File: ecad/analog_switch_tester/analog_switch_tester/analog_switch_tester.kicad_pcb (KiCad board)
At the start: 2 copper layers, 5 parts, among them J1 Conn_01x03_Pin, U1 DRV5056A1xQDBZxR

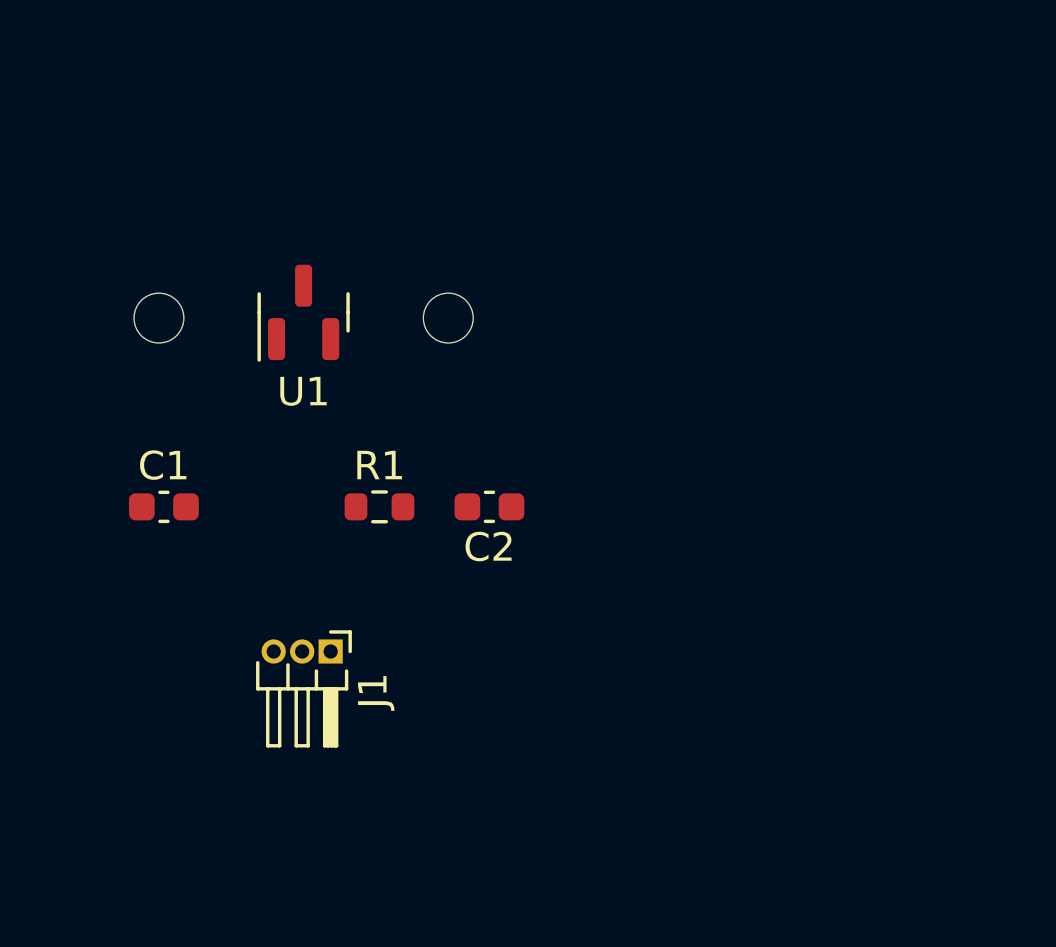
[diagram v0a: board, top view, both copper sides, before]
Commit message: .
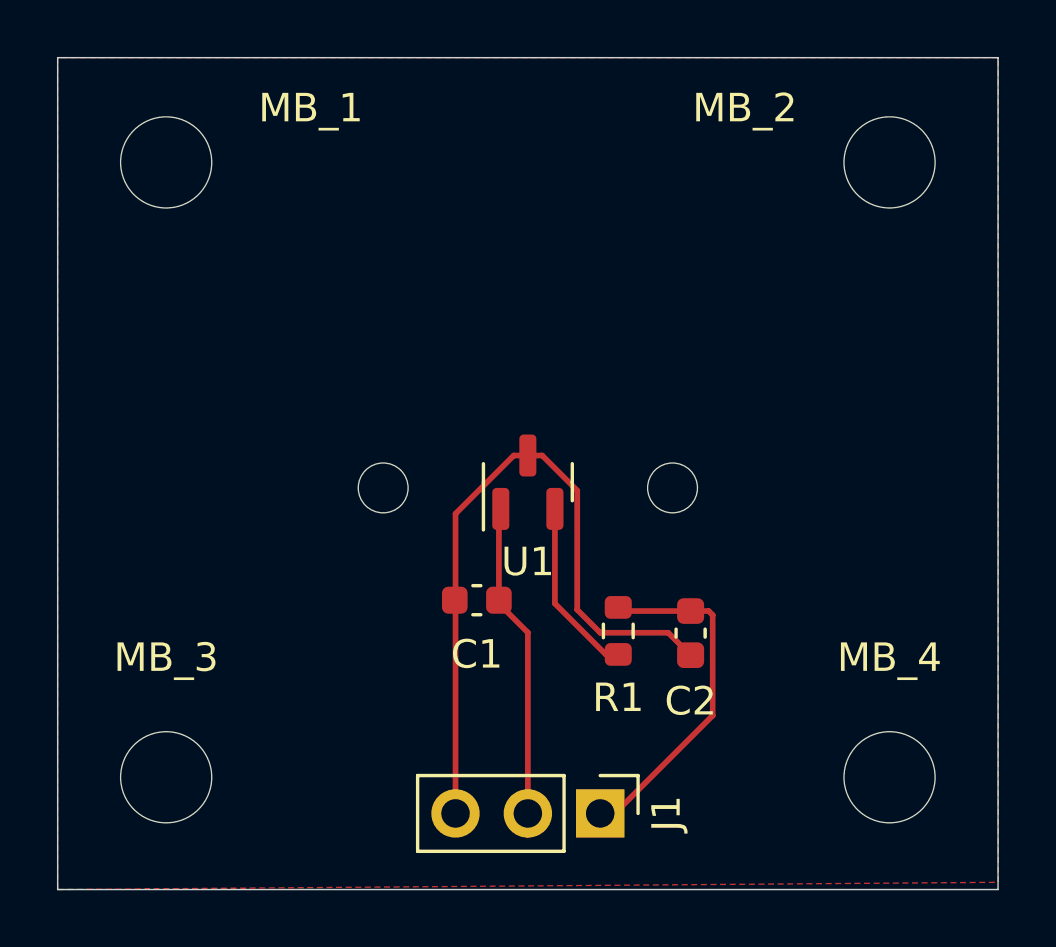
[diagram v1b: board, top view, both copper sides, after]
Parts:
- added MB_1: MountingHole_3.2mm_M3, MountingHole:MountingHole_3.2mm_M3, F.Cu at (23.1, 22.5)
- added MB_2: MountingHole_3.2mm_M3, MountingHole:MountingHole_3.2mm_M3, F.Cu at (48.5, 22.5)
- added MB_3: MountingHole_3.2mm_M3, MountingHole:MountingHole_3.2mm_M3, F.Cu at (23.1, 44.1)
- added MB_4: MountingHole_3.2mm_M3, MountingHole:MountingHole_3.2mm_M3, F.Cu at (48.5, 44.1)
- J1: footprint Connector_PinHeader_1.00mm:PinHeader_1x03_P1.00mm_Horizontal -> Connector_PinHeader_2.54mm:PinHeader_1x03_P2.54mm_Vertical
- moved C1 11.5 mm to (34.0, 37.8)
- moved J1 11.0 mm to (38.4, 45.3)
- moved U1 9.88 mm to (35.8, 33.9)
- moved R1 9.45 mm to (39.0, 38.9), turned to 90 degrees
- moved C2 8.34 mm to (41.5, 39.0), turned to 90 degrees
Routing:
- net GNDA: track 0.00 -> 25.4 mm
- net OUT: track 0.00 -> 12.4 mm
- net V_AREF: track 0.00 -> 11.9 mm
- net Net-(U1-OUT): track 0.00 -> 6.30 mm
- added copper zone on F.Cu, net GNDA
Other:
- board outline added: 33 x 29.2 mm
